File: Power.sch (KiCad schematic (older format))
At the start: 90 parts

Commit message: update
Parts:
- removed C?: 10uF/6.3V/20%/X5R/C0603, OLIMEX_RLC-FP:C_0603_5MIL_DWS, symbol S3-OLinuXino_Rev_A:C
- removed C?: 47uF/6.3V/20%/X5R/C0805, OLIMEX_RLC-FP:C_0805_5MIL_DWS, symbol S3-OLinuXino_Rev_A:C
- removed D? (x2): 1N5822/SS34/SMA, OLIMEX_Diodes-FP:SMA-KA, symbol S3-OLinuXino_Rev_A:D_Schottky
- removed FET?: IRLML6402(SOT-23), OLIMEX_Transistors-FP:SOT23, symbol S3-OLinuXino_Rev_A:P-MOS+DIOD
- removed L?: 2.2uH/4.5A/28mR/20%/CD75/7.8x7.0x5.0mm(YS75-2R2M), OLIMEX_RLC-FP:YS75_7X8MM, symbol S3-OLinuXino_Rev_A:L
- removed PWRLED?: LED\\Red\\0603, OLIMEX_LEDs-FP:LED_0603_KA, symbol S3-OLinuXino_Rev_A:LED
- removed R?: 2.2k/R0402, OLIMEX_RLC-FP:R_0402_5MIL_DWS, symbol S3-OLinuXino_Rev_A:R
- removed R?: 1.1k/1%/R0402, OLIMEX_RLC-FP:R_0402_5MIL_DWS, symbol S3-OLinuXino_Rev_A:R
- removed R?: 8.25k/1%/R0402, OLIMEX_RLC-FP:R_0402_5MIL_DWS, symbol S3-OLinuXino_Rev_A:R
- removed R?: 10k/R0402, OLIMEX_RLC-FP:R_0402_5MIL_DWS, symbol S3-OLinuXino_Rev_A:R
- removed U?: MT3608(SOT23-6), OLIMEX_IC-FP:SOT23-6, symbol S3-OLinuXino_Rev_A:MT3608(SOT23-6)
- added D?: LED, symbol Device:LED
- added R?: 5k1, otter:C_0402, symbol Device:R_Small
- added R? (x2): DNP, otter:C_0402, symbol Device:R_Small
- J?: value USB_C_Receptacle_USB2.0 -> USB
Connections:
- net labels removed: +5V_EXT
- wire segments 362 -> 326
- no-connect marks 6 -> 8
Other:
- note removed: "DELETE?\nMacht 5V ext aus batt"
- note removed: "Ra"
- note removed: "Rb"
- note removed: "Vout=0.6*(1+Ra\Rb)"
- moved on the sheet: C?, J?, L?, R?, U?

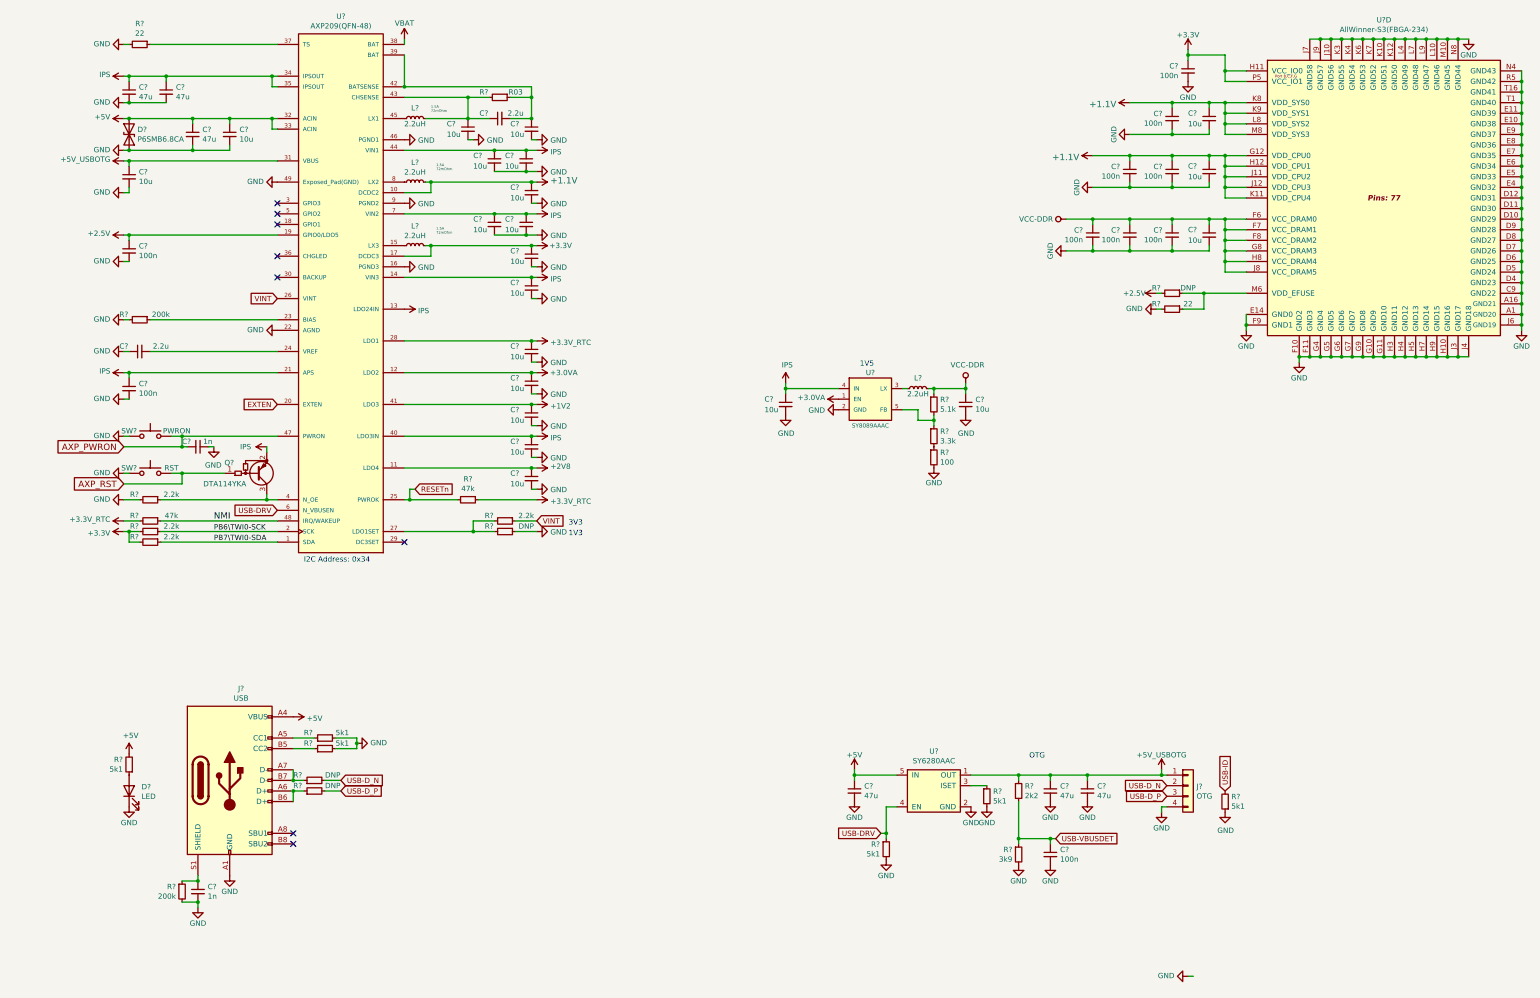
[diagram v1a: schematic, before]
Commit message: update
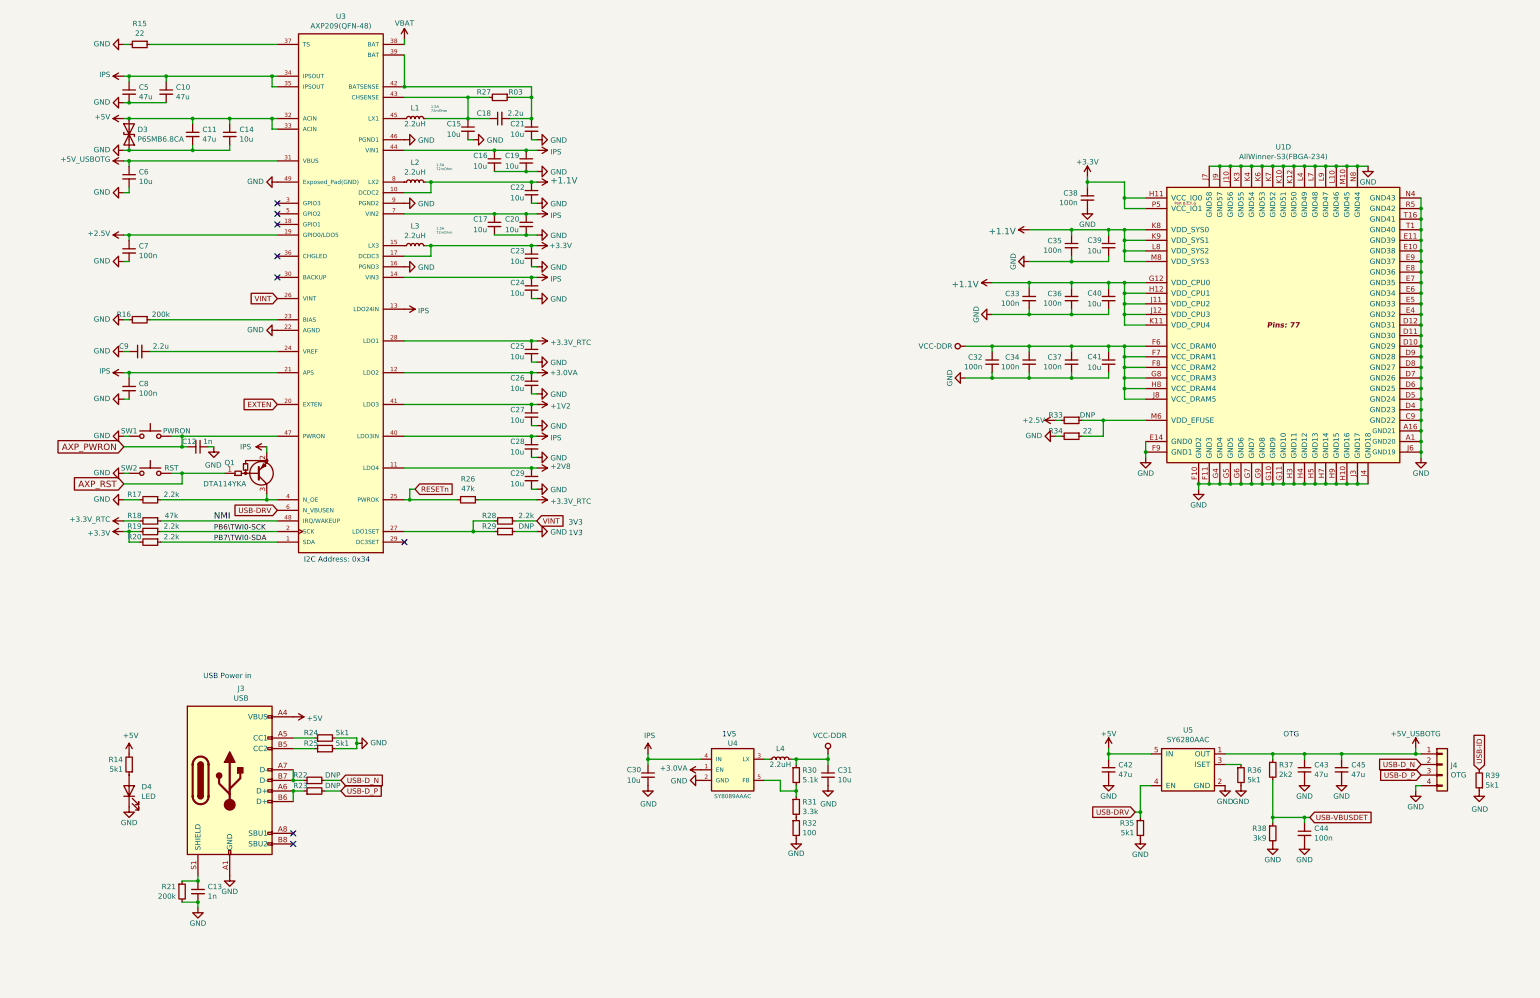
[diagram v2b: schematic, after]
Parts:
- gave numbers to parts that had none: 82
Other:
- note added: "USB Power in"
- moved on the sheet: C30, C31, C32, C33, C34, C35, C36, C37, C38, C39, C40, C41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

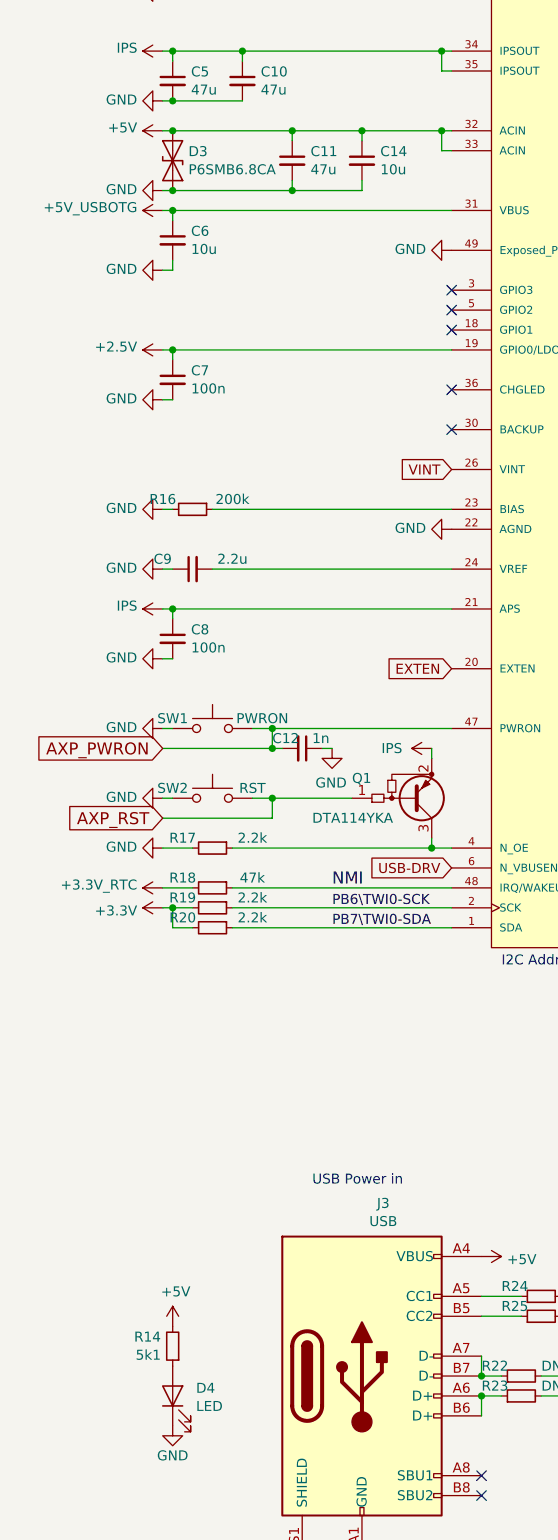
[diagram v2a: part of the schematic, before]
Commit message: update
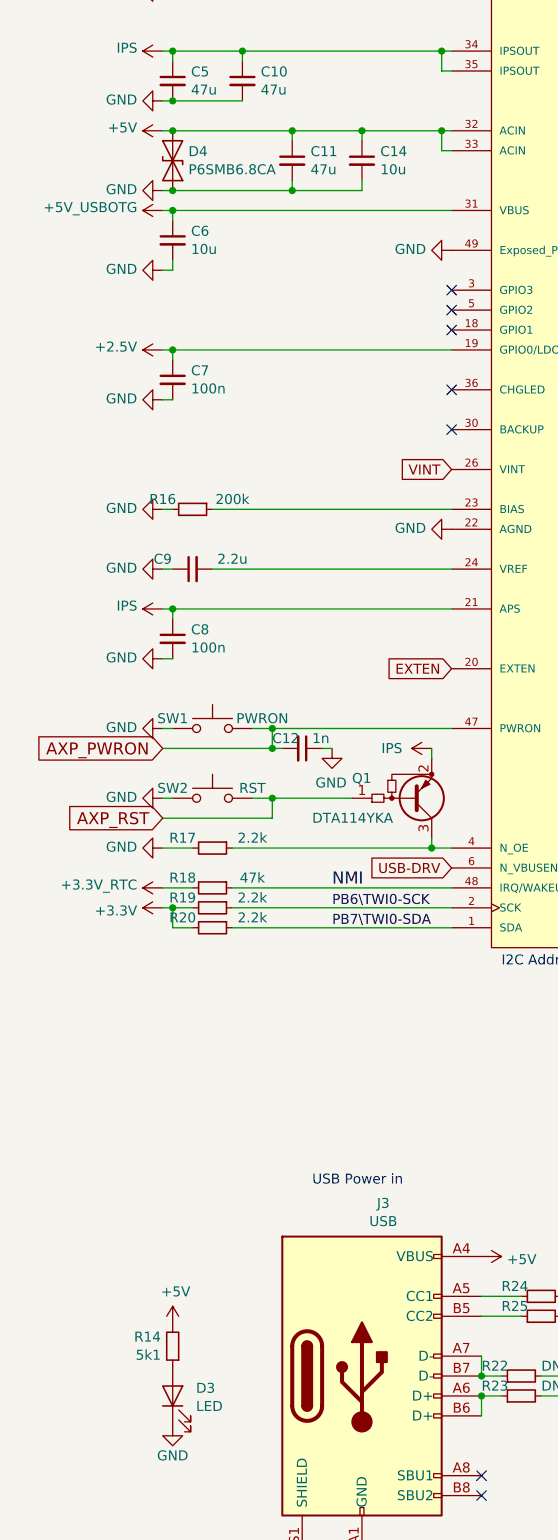
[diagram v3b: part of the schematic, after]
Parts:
- D3: renamed from D4; footprint (none) -> otter:LED_0603_1608Metric
- D4: renamed from D3; footprint (none) -> Diode_SMD:D_SMB
- J3: footprint (none) -> otter:USB-C 16Pin
- J4: footprint (none) -> Connector_PinHeader_2.00mm:PinHeader_1x04_P2.00mm_Vertical
- L1, L2, L3, L4: footprint (none) -> Inductor_SMD:L_Taiyo-Yuden_MD-3030
- Q1: footprint (none) -> Package_TO_SOT_SMD:SOT-23
- SW1, SW2: footprint (none) -> Button_Switch_SMD:SW_SPST_PTS810
- U1: footprint OLIMEX_IC-FP:FBGA-234(Pitch-0.65mm_Pad-0.3mm_11x11x1.08mm) -> otter:FBGA-234(Pitch-0.65mm_Pad-0.3mm_11x11x1.08mm)
- U3: footprint OLIMEX_IC-FP:QFN48-6x6mm-OLIMEX_V2 -> otter:QFN-48-1EP_6x6mm_P0.4mm_EP4.05x4.05mm
- U4: footprint OLIMEX_Regulators-FP:SOT-23-5 -> Package_TO_SOT_SMD:SOT-23-5
- U5: footprint (none) -> Package_TO_SOT_SMD:SOT-23-5
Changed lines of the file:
@@
 F 0 "U4" H 7550 8350 50  0000 C CNN
 F 1 "SY8089AAAC" H 7550 7850 39  0000 C CNN
-F 2 "OLIMEX_Regulators-FP:SOT-23-5" H 7580 8250 20  0001 C CNN
+F 2 "Package_TO_SOT_SMD:SOT-23-5" H 7580 8250 20  0001 C CNN
 F 3 "" H 7550 8100 60  0000 C CNN
 F 4 "Value 1" H 7550 8100 60  0001 C CNN "Fieldname 1"
@@
 F 0 "L3" V 4735 3150 50  0000 C CNN
 F 1 "2.2uH" V 4644 3150 50  0000 C CNN
-F 2 "" H 4550 3150 50  0001 C CNN
+F 2 "Inductor_SMD:L_Taiyo-Yuden_MD-3030" H 4550 3150 50  0001 C CNN
 F 3 "~" H 4550 3150 50  0001 C CNN
 	1    4550 3150
@@
 F 0 "L2" V 4735 2550 50  0000 C CNN
 F 1 "2.2uH" V 4644 2550 50  0000 C CNN
-F 2 "" H 4550 2550 50  0001 C CNN
+F 2 "Inductor_SMD:L_Taiyo-Yuden_MD-3030" H 4550 2550 50  0001 C CNN
 F 3 "~" H 4550 2550 50  0001 C CNN
 	1    4550 2550
@@
 F 0 "L1" V 4650 1950 50  0000 C CNN
 F 1 "2.2uH" V 4500 1950 50  0000 C CNN
-F 2 "" H 4550 1950 50  0001 C CNN
+F 2 "Inductor_SMD:L_Taiyo-Yuden_MD-3030" H 4550 1950 50  0001 C CNN
 F 3 "~" H 4550 1950 50  0001 C CNN
 	1    4550 1950
@@
 F 0 "Q1" H 2750 5200 50  0000 L CNN
 F 1 "DTA114YKA" H 2550 5400 50  0000 L CNN
-F 2 "" H 3100 5300 50  0001 C CNN
+F 2 "Package_TO_SOT_SMD:SOT-23" H 3100 5300 50  0001 C CNN
 F 3 "~" H 3100 5300 50  0001 C CNN
 	1    3100 5300
@@
 F 0 "SW2" H 1850 5350 50  0000 C CNN
 F 1 "RST" H 2250 5350 50  0000 C CNN
-F 2 "" H 2050 5500 50  0001 C CNN
+F 2 "Button_Switch_SMD:SW_SPST_PTS810" H 2050 5500 50  0001 C CNN
 F 3 "~" H 2050 5500 50  0001 C CNN
 	1    2050 5300
@@
 	1800 2350 1850 2350
 $Comp
-L Device:D_TVS D3
+L Device:D_TVS D4
 U 1 1 66BA7290
 P 1850 2100
-F 0 "D3" V 1804 2179 50  0000 L CNN
+F 0 "D4" V 1804 2179 50  0000 L CNN
 F 1 "P6SMB6.8CA" V 1895 2179 50  0000 L CNN
-F 2 "" H 1850 2100 50  0001 C CNN
+F 2 "Diode_SMD:D_SMB" H 1850 2100 50  0001 C CNN
 F 3 "~" H 1850 2100 50  0001 C CNN
 	1    1850 2100
@@
 F 0 "SW1" H 1850 5000 50  0000 C CNN
 F 1 "PWRON" H 2300 5000 50  0000 C CNN
-F 2 "" H 2050 5150 50  0001 C CNN
+F 2 "Button_Switch_SMD:SW_SPST_PTS810" H 2050 5150 50  0001 C CNN
 F 3 "~" H 2050 5150 50  0001 C CNN
 	1    2050 4950
@@
 F 0 "L4" V 8100 8000 50  0000 C CNN
 F 1 "2.2uH" V 7950 8000 50  0000 C CNN
-F 2 "" H 8000 8000 50  0001 C CNN
+F 2 "Inductor_SMD:L_Taiyo-Yuden_MD-3030" H 8000 8000 50  0001 C CNN
 F 3 "~" H 8000 8000 50  0001 C CNN
 	1    8000 8000
@@
 F 0 "U3" H 3850 6115 50  0000 C CNN
 F 1 "AXP209(QFN-48)" H 3850 6024 50  0000 C CNN
-F 2 "OLIMEX_IC-FP:QFN48-6x6mm-OLIMEX_V2" H 3850 850 50  0001 C CNN
+F 2 "otter:QFN-48-1EP_6x6mm_P0.4mm_EP4.05x4.05mm" H 3850 850 50  0001 C CNN
 F 3 "http://dl.linux-sunxi.org/AXP/AXP209_Datasheet_v1.0en.pdf" H 3850 750 50  0001 C CNN
 	1    3850 3550
@@
 F 0 "U1" H 12750 5581 50  0000 C CNN
 F 1 "AllWinner-S3(FBGA-234)" H 12750 5490 50  0000 C CNN
-F 2 "OLIMEX_IC-FP:FBGA-234(Pitch-0.65mm_Pad-0.3mm_11x11x1.08mm)" H 12750 1850 50  0001 C CNN
+F 2 "otter:FBGA-234(Pitch-0.65mm_Pad-0.3mm_11x11x1.08mm)" H 12750 1850 50  0001 C CNN
 F 3 "" H 12950 5600 50  0001 C CNN
 	4    12750 3900
@@
 F 0 "U5" H 11850 8475 50  0000 C CNN
 F 1 "SY6280AAC" H 11850 8384 50  0000 C CNN
-F 2 "" H 11850 8100 50  0001 C CNN
+F 2 "Package_TO_SOT_SMD:SOT-23-5" H 11850 8100 50  0001 C CNN
 F 3 "" H 11850 8100 50  0001 C CNN
 	1    11850 8100
@@
 F 0 "J4" H 14330 8042 50  0000 L CNN
 F 1 "OTG" H 14330 7951 50  0000 L CNN
-F 2 "" H 14250 8050 50  0001 C CNN
+F 2 "Connector_PinHeader_2.00mm:PinHeader_1x04_P2.00mm_Vertical" H 14250 8050 50  0001 C CNN
 F 3 "~" H 14250 8050 50  0001 C CNN
 	1    14250 8050
@@
 F 0 "J3" H 2907 9067 50  0000 C CNN
 F 1 "USB" H 2907 8976 50  0000 C CNN
-F 2 "" H 2950 8200 50  0001 C CNN
+F 2 "otter:USB-C 16Pin" H 2950 8200 50  0001 C CNN
 F 3 "https://www.usb.org/sites/default/files/documents/usb_type-c.zip" H 2950 8200 50  0001 C CNN
 	1    2800 8200
@@
 P 1850 8300
 AR Path="/5FC342C2" Ref="D?"  Part="1"
-AR Path="/602ACDF9/5FC342C2" Ref="D4"  Part="1"
-F 0 "D4" V 1889 8183 50  0000 R CNN
+AR Path="/602ACDF9/5FC342C2" Ref="D3"  Part="1"
+F 0 "D3" V 1889 8183 50  0000 R CNN
 F 1 "LED" V 1798 8183 50  0000 R CNN
-F 2 "" H 1850 8300 50  0001 C CNN
+F 2 "otter:LED_0603_1608Metric" H 1850 8300 50  0001 C CNN
 F 3 "~" H 1850 8300 50  0001 C CNN
 	1    1850 8300
